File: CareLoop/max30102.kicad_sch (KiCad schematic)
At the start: 10 parts, among them U1 MCP1700x-180xxMB, U2 MAX30102

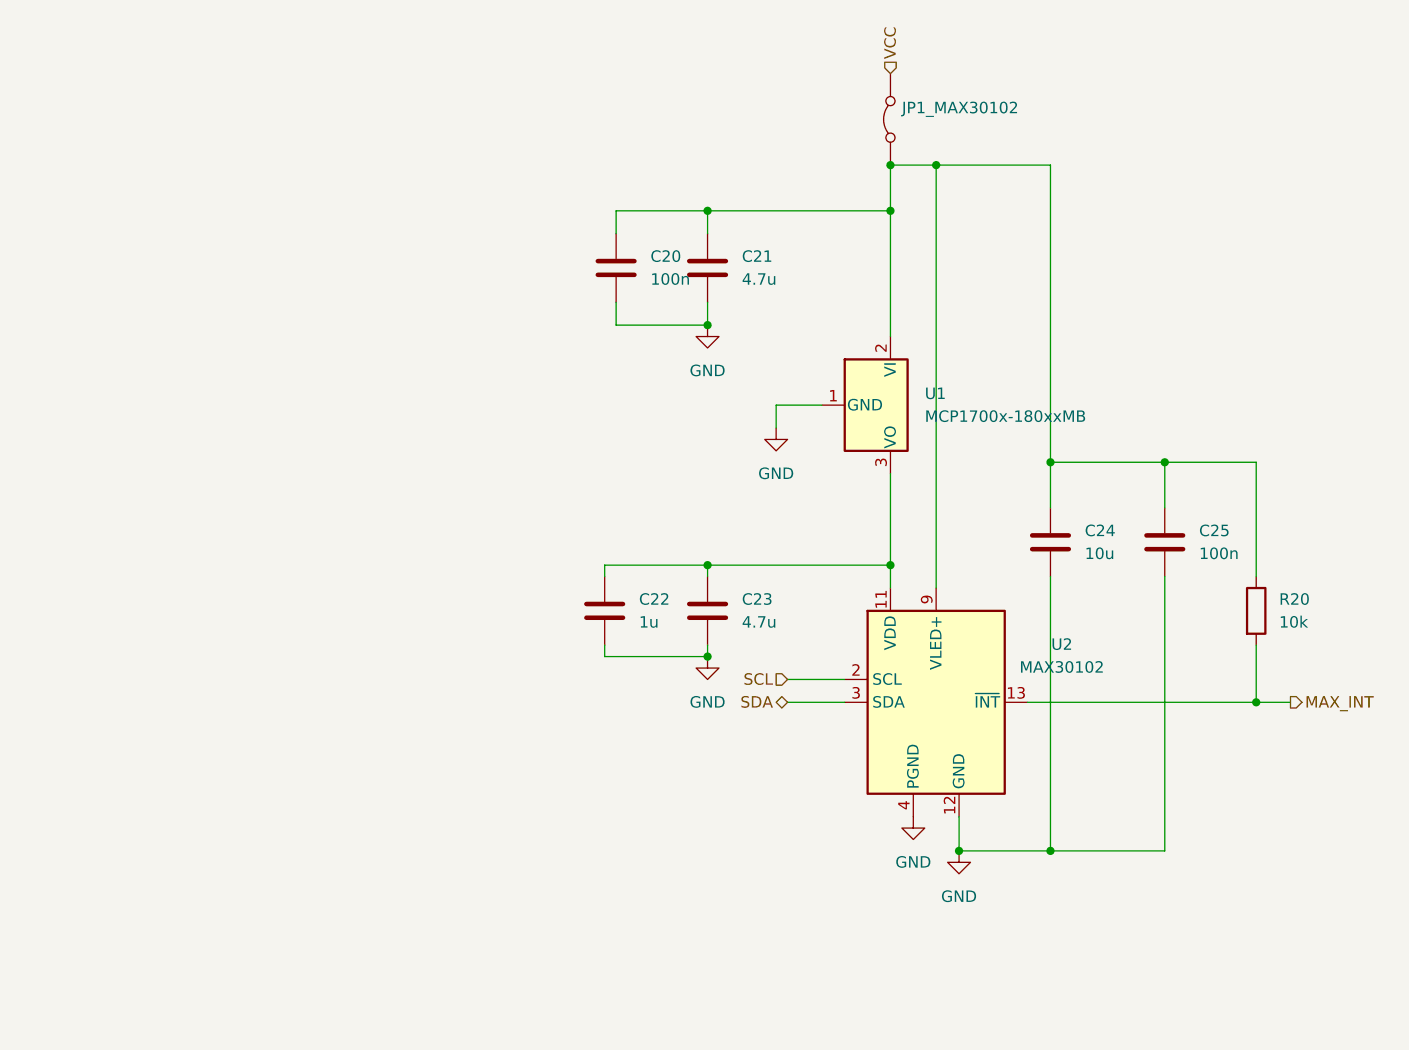
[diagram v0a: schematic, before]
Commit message: WP: updatet version with routing
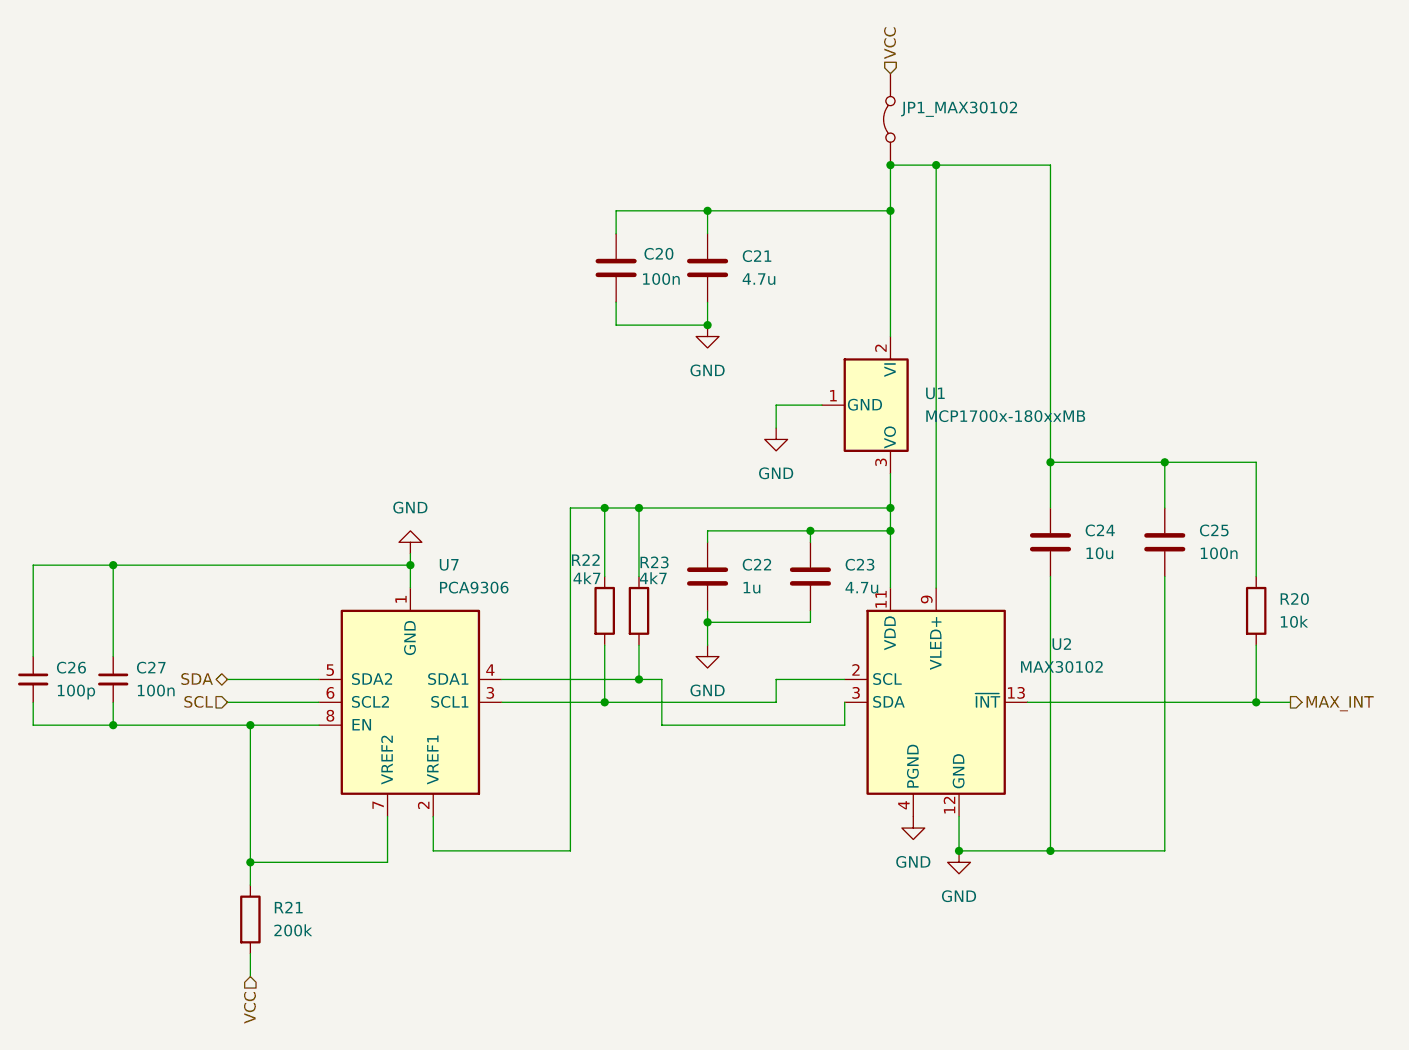
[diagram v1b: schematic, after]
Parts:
- added C26: 100p, Capacitor_SMD:C_0201_0603Metric_Pad0.64x0.40mm_HandSolder, symbol Device:C_Small
- added C27: 100n, Capacitor_SMD:C_0201_0603Metric_Pad0.64x0.40mm_HandSolder, symbol Device:C_Small
- added R21: 200k, Resistor_SMD:R_0402_1005Metric_Pad0.72x0.64mm_HandSolder, symbol Device:R
- added R22, R23: 4k7, Resistor_SMD:R_0402_1005Metric_Pad0.72x0.64mm_HandSolder, symbol Device:R
- added U7: PCA9306, Package_SON:X2SON-8_1.4x1mm_P0.35mm, symbol Interface:PCA9306
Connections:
- net GND: now also C26.1, C27.1, U7.1 (GND)
- net SCL: now also U7.6 (SCL2); no longer U2.2 (SCL)
- net SDA: now also U7.5 (SDA2); no longer U2.3 (SDA)
- net VCC: now also R21.2
- net at C22.1, C23.1, U1.3 (VO)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: now also R22.1, R23.1, U7.2 (VREF1)
- new net: C26.2, C27.2, R21.1, U7.7 (VREF2), U7.8 (EN)
- new net: R22.2, U2.2 (SCL), U7.3 (SCL1)
- new net: R23.2, U2.3 (SDA), U7.4 (SDA1)
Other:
- moved on the sheet: C22, C23
